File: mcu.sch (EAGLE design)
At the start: 49 parts, among them IC1 MCP73831/OT, SW1 MF-SW-TACT-4.2MM, T1 SI7051-A20, U1 MF-REG-SOT235-3.3V-300mA, U4 NRF52832, X1 LFXTAL069526, X6 32.768kHz

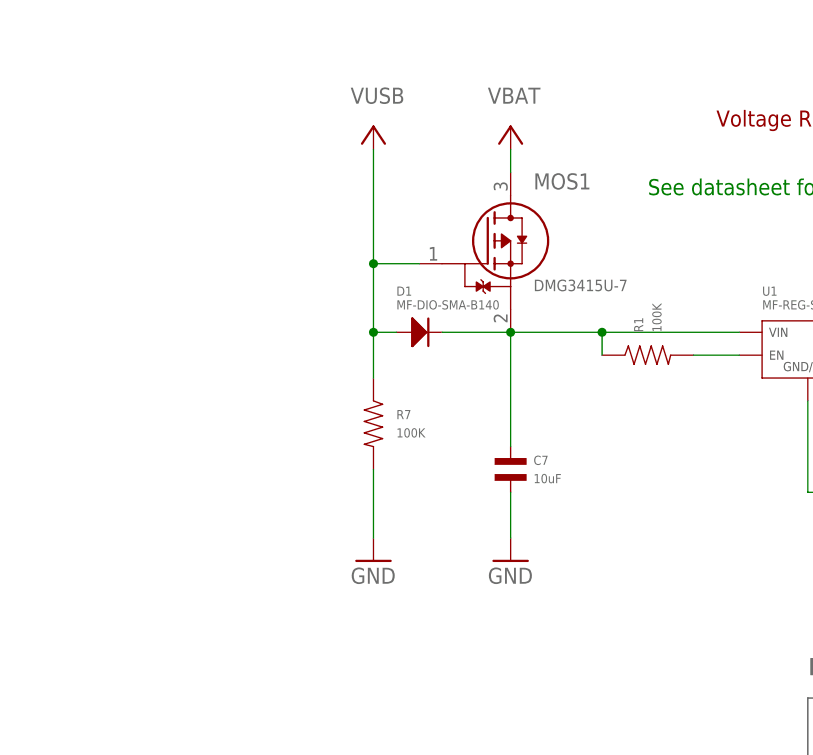
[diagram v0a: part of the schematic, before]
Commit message: UPD: finished design for v2, submitted to macrofab
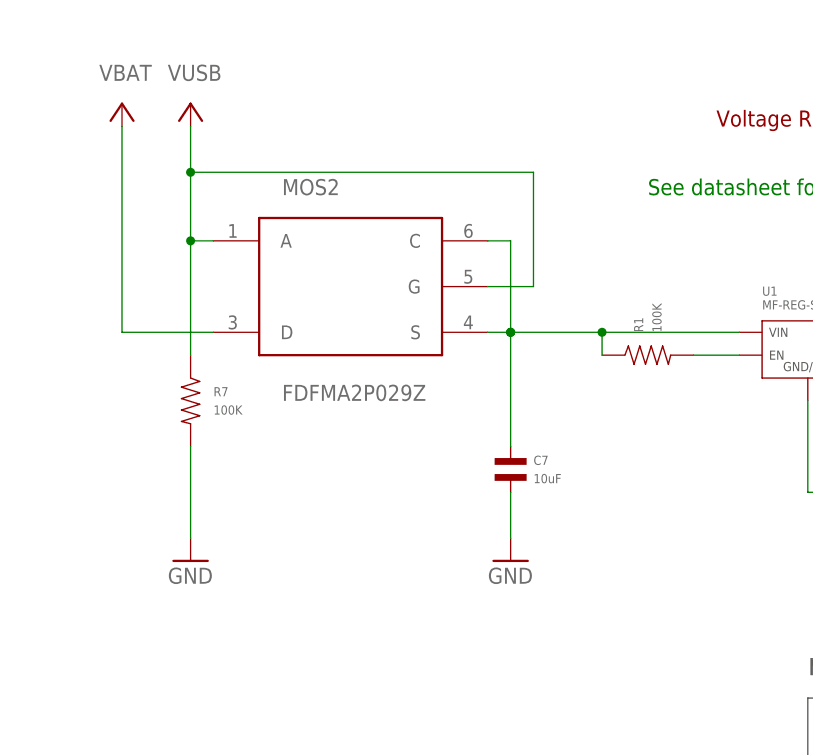
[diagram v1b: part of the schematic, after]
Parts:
- removed D1: MF-DIO-SMA-B140, MF_Discrete_Semiconductor:DIODES_B140_SMA
- removed MOS1: DMG3415U-7, tilesPartComp:DMG3415U-7
- added MOS2: FDFMA2P029Z, tilesPartComp:FDFMA2P029Z
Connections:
- removed net N$2: C7.P$1, D1.CATHODE, MOS1.S, R1.P$1, U1.VIN
- new net N$12: C7.P$1, MOS2.C, MOS2.S, R1.P$1, U1.VIN
- net VBAT: now also MOS2.D; no longer MOS1.D
- net VUSB: now also MOS2.A, MOS2.G; no longer D1.ANODE, MOS1.G
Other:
- moved on the sheet: R7
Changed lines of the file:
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@@
 <part name="VDD_3" library="supply2" library_urn="urn:adsk.eagle:library:372" deviceset="V+" device="" value="3.3V"/>
 <part name="VDD_4" library="supply2" library_urn="urn:adsk.eagle:library:372" deviceset="V+" device="" value="3.3V"/>
-<part name="U$2" library="tilesPartComp" deviceset="VBAT" device=""/>
-<part name="U$3" library="tilesPartComp" deviceset="VUSB" device=""/>
-<part name="MOS1" library="tilesPartComp" deviceset="DMG3415U" device="" technology="-7">
-<attribute name="MPN" value="DMG3415U-7"/>
-</part>
-<part name="D1" library="MF_Discrete_Semiconductor" deviceset="DIODES" device="_SMA" technology="_B140" value="MF-DIO-SMA-B140"/>
 <part name="USB1" library="tilesPartComp" deviceset="ZX62R-B-5P(30)" device="">
 <attribute name="MPN" value="ZX62R-B-5P(30)"/>
@@
 <attribute name="MPN" value="MF-IND-1210-10uH"/>
 </part>
+<part name="MOS2" library="tilesPartComp" deviceset="FDFMA2P029Z" device="">
+<attribute name="MPN" value="FDFMA2P029Z"/>
+</part>
+<part name="U$1" library="tilesPartComp" deviceset="VBAT" device=""/>
+<part name="U$7" library="tilesPartComp" deviceset="VUSB" device=""/>
 </parts>
 <sheets>
@@
 <attribute name="MPN" x="68.58" y="226.06" size="1.778" layer="96" display="off"/>
 </instance>
-<instance part="GND1" gate="1" x="-81.28" y="320.04"/>
+<instance part="GND1" gate="1" x="-101.6" y="320.04"/>
 <instance part="GND2" gate="1" x="-66.04" y="320.04"/>
 <instance part="GND4" gate="1" x="-5.08" y="320.04"/>
@@
 <instance part="VDD_3" gate="1" x="38.1" y="195.58"/>
 <instance part="VDD_4" gate="1" x="-5.08" y="368.3"/>
-<instance part="U$2" gate="G$1" x="-66.04" y="368.3"/>
-<instance part="U$3" gate="G$2" x="-81.28" y="368.3"/>
-<instance part="MOS1" gate="DMG3415U*" x="-68.58" y="355.6">
-<attribute name="MPN" x="-68.58" y="355.6" size="1.778" layer="96" display="off"/>
-</instance>
-<instance part="D1" gate="G$1" x="-76.2" y="345.44"/>
 <instance part="USB1" gate="ZX62R-B-5P(30)" x="45.72" y="355.6">
 <attribute name="MPN" x="45.72" y="355.6" size="1.778" layer="96" display="off"/>
@@
 <attribute name="MPN" x="10.16" y="106.68" size="1.778" layer="96" display="off"/>
 </instance>
-<instance part="R7" gate="G$1" x="-81.28" y="335.28"/>
+<instance part="R7" gate="G$1" x="-101.6" y="337.82"/>
 <instance part="R1" gate="G$1" x="-50.8" y="342.9" rot="R90"/>
 <instance part="C7" gate="G$1" x="-66.04" y="330.2"/>
@@
 <instance part="C9" gate="G$1" x="68.58" y="294.64"/>
 <instance part="L1" gate="G$1" x="53.34" y="274.32" rot="R90"/>
+<instance part="MOS2" gate="G$1" x="-83.82" y="350.52">
+<attribute name="MPN" x="-83.82" y="350.52" size="1.778" layer="96" display="off"/>
+</instance>
+<instance part="U$1" gate="G$1" x="-109.22" y="370.84"/>
+<instance part="U$7" gate="G$2" x="-101.6" y="370.84"/>
 </instances>
 <busses>
@@
 <pinref part="R7" gate="G$1" pin="P$2"/>
 <pinref part="GND1" gate="1" pin="GND"/>
-<wire x1="-81.28" y1="330.2" x2="-81.28" y2="322.58" width="0.1524" layer="91"/>
+<wire x1="-101.6" y1="332.74" x2="-101.6" y2="322.58" width="0.1524" layer="91"/>
 </segment>
 <segment>
@@
 </segment>
 </net>
-<net name="N$2" class="0">
-<segment>
-<wire x1="-66.04" y1="345.44" x2="-55.88" y2="345.44" width="0.1524" layer="91"/>
-<pinref part="MOS1" gate="DMG3415U*" pin="S"/>
-<wire x1="-55.88" y1="345.44" x2="-40.64" y2="345.44" width="0.1524" layer="91"/>
-<wire x1="-66.04" y1="332.74" x2="-66.04" y2="345.44" width="0.1524" layer="91"/>
-<junction x="-66.04" y="345.44"/>
-<pinref part="D1" gate="G$1" pin="CATHODE"/>
-<wire x1="-73.66" y1="345.44" x2="-66.04" y2="345.44" width="0.1524" layer="91"/>
-<pinref part="R1" gate="G$1" pin="P$1"/>
-<wire x1="-55.88" y1="342.9" x2="-55.88" y2="345.44" width="0.1524" layer="91"/>
-<junction x="-55.88" y="345.44"/>
-<pinref part="C7" gate="G$1" pin="P$1"/>
-<pinref part="U1" gate="G$1" pin="VIN"/>
-</segment>
-</net>
 <net name="USBD-" class="0">
 <segment>
@@
 </net>
 <net name="VBAT" class="0">
-<segment>
-<pinref part="MOS1" gate="DMG3415U*" pin="D"/>
-<pinref part="U$2" gate="G$1" pin="VBAT"/>
-<wire x1="-66.04" y1="363.22" x2="-66.04" y2="365.76" width="0.1524" layer="91"/>
-</segment>
 <segment>
 <pinref part="U$6" gate="G$1" pin="VBAT"/>
@@
 <wire x1="-53.34" y1="236.22" x2="-53.34" y2="248.92" width="0.1524" layer="91"/>
 </segment>
+<segment>
+<pinref part="U$1" gate="G$1" pin="VBAT"/>
+<pinref part="MOS2" gate="G$1" pin="D"/>
+<wire x1="-109.22" y1="368.3" x2="-109.22" y2="345.44" width="0.1524" layer="91"/>
+<wire x1="-109.22" y1="345.44" x2="-99.06" y2="345.44" width="0.1524" layer="91"/>
+</segment>
 </net>
 <net name="VUSB" class="0">
-<segment>
-<pinref part="U$3" gate="G$2" pin="VUSB"/>
-<pinref part="MOS1" gate="DMG3415U*" pin="G"/>
-<wire x1="-81.28" y1="345.44" x2="-81.28" y2="353.06" width="0.1524" layer="91"/>
-<wire x1="-81.28" y1="353.06" x2="-81.28" y2="365.76" width="0.1524" layer="91"/>
-<wire x1="-76.2" y1="353.06" x2="-81.28" y2="353.06" width="0.1524" layer="91"/>
-<junction x="-81.28" y="353.06"/>
-<pinref part="D1" gate="G$1" pin="ANODE"/>
-<wire x1="-78.74" y1="345.44" x2="-81.28" y2="345.44" width="0.1524" layer="91"/>
-<pinref part="R7" gate="G$1" pin="P$1"/>
-<wire x1="-81.28" y1="345.44" x2="-81.28" y2="340.36" width="0.1524" layer="91"/>
-<junction x="-81.28" y="345.44"/>
-</segment>
 <segment>
 <pinref part="U$4" gate="G$2" pin="VUSB"/>
@@
 <pinref part="D3" gate="G$1" pin="ANODE"/>
 </segment>
+<segment>
+<pinref part="U$7" gate="G$2" pin="VUSB"/>
+<wire x1="-101.6" y1="368.3" x2="-101.6" y2="363.22" width="0.1524" layer="91"/>
+<pinref part="MOS2" gate="G$1" pin="G"/>
+<wire x1="-63.5" y1="363.22" x2="-63.5" y2="350.52" width="0.1524" layer="91"/>
+<wire x1="-63.5" y1="350.52" x2="-68.58" y2="350.52" width="0.1524" layer="91"/>
+<wire x1="-63.5" y1="363.22" x2="-101.6" y2="363.22" width="0.1524" layer="91"/>
+<pinref part="R7" gate="G$1" pin="P$1"/>
+<wire x1="-101.6" y1="363.22" x2="-101.6" y2="355.6" width="0.1524" layer="91"/>
+<junction x="-101.6" y="363.22"/>
+<pinref part="MOS2" gate="G$1" pin="A"/>
+<wire x1="-101.6" y1="355.6" x2="-101.6" y2="342.9" width="0.1524" layer="91"/>
+<wire x1="-99.06" y1="355.6" x2="-101.6" y2="355.6" width="0.1524" layer="91"/>
+<junction x="-101.6" y="355.6"/>
+</segment>
 </net>
 <net name="N$1" class="0">
@@
 </segment>
 </net>
+<net name="N$12" class="0">
+<segment>
+<pinref part="MOS2" gate="G$1" pin="C"/>
+<wire x1="-68.58" y1="355.6" x2="-66.04" y2="355.6" width="0.1524" layer="91"/>
+<wire x1="-66.04" y1="355.6" x2="-66.04" y2="345.44" width="0.1524" layer="91"/>
+<pinref part="MOS2" gate="G$1" pin="S"/>
+<wire x1="-66.04" y1="345.44" x2="-68.58" y2="345.44" width="0.1524" layer="91"/>
+<junction x="-66.04" y="345.44"/>
+<wire x1="-66.04" y1="345.44" x2="-55.88" y2="345.44" width="0.1524" layer="91"/>
+<wire x1="-55.88" y1="345.44" x2="-40.64" y2="345.44" width="0.1524" layer="91"/>
+<wire x1="-66.04" y1="332.74" x2="-66.04" y2="345.44" width="0.1524" layer="91"/>
+<pinref part="R1" gate="G$1" pin="P$1"/>
+<wire x1="-55.88" y1="342.9" x2="-55.88" y2="345.44" width="0.1524" layer="91"/>
+<junction x="-55.88" y="345.44"/>
+<pinref part="C7" gate="G$1" pin="P$1"/>
+<pinref part="U1" gate="G$1" pin="VIN"/>
+<junction x="-66.04" y="345.44"/>
+</segment>
+</net>
